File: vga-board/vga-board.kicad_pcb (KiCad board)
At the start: 2 copper layers, 141 x 95.2 mm, 44 parts, among them J1 Conn_02x20_Odd_Even, J2 Conn_02x20_Odd_Even, J3 DB15_Female_HighDensity, U1 74HC244, U10 74HC163, U11 74LS158, U12 74LS251, U13 74HC244, U14 74HC244, U15 74HC244, U16 GAL22V10, U17 GAL22V10, U18 GAL22V10, U19 74HC163, U2 74HC373, U20 74HC163, U21 74HC163, U22 74HC163, U23 74HC163, U3 74HC244, U4 74HC373, U5 74HC373, U6 74HC373, U7 74HC373, U8 71256SA12TPG, U9 74HC244, X1 40MHz

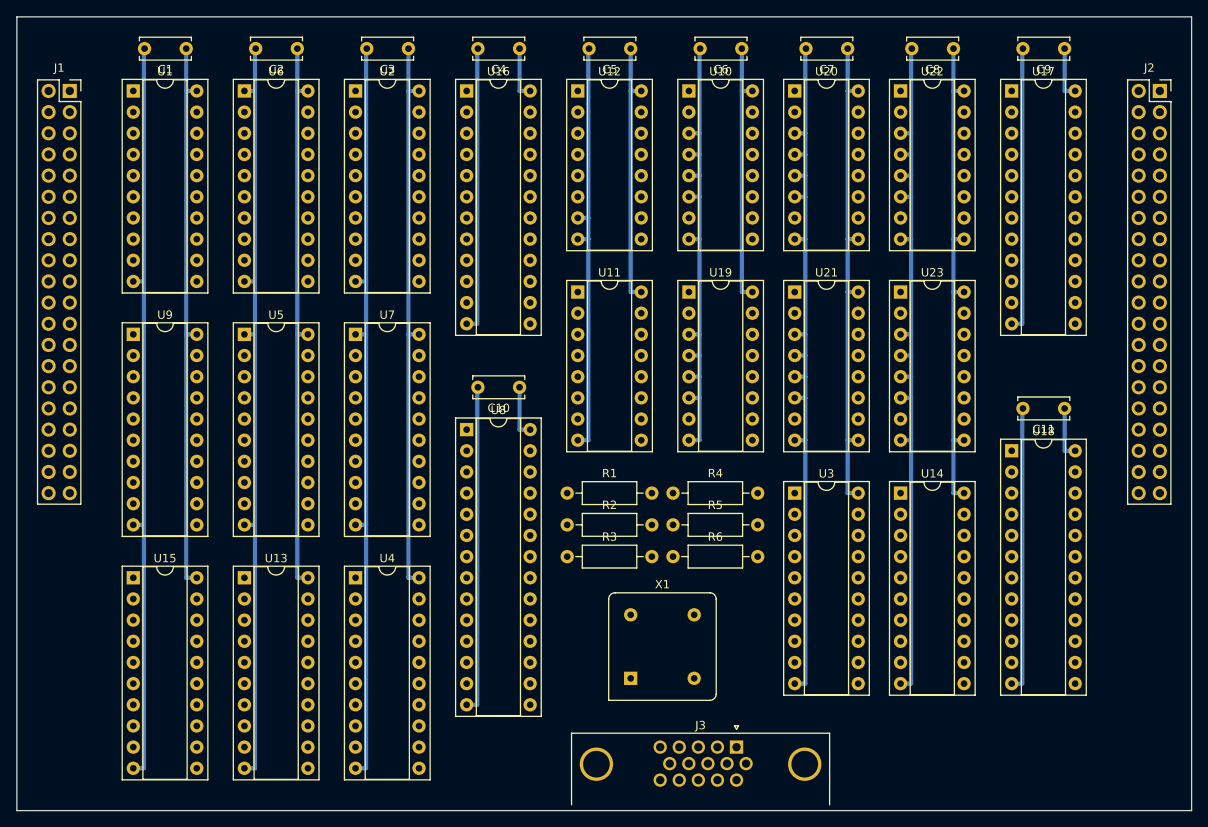
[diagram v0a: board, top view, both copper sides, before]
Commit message: Revert "More on layouts"
This reverts commit 3fc7c4d1a32f245eaa0a26aebed00be081417dbd.
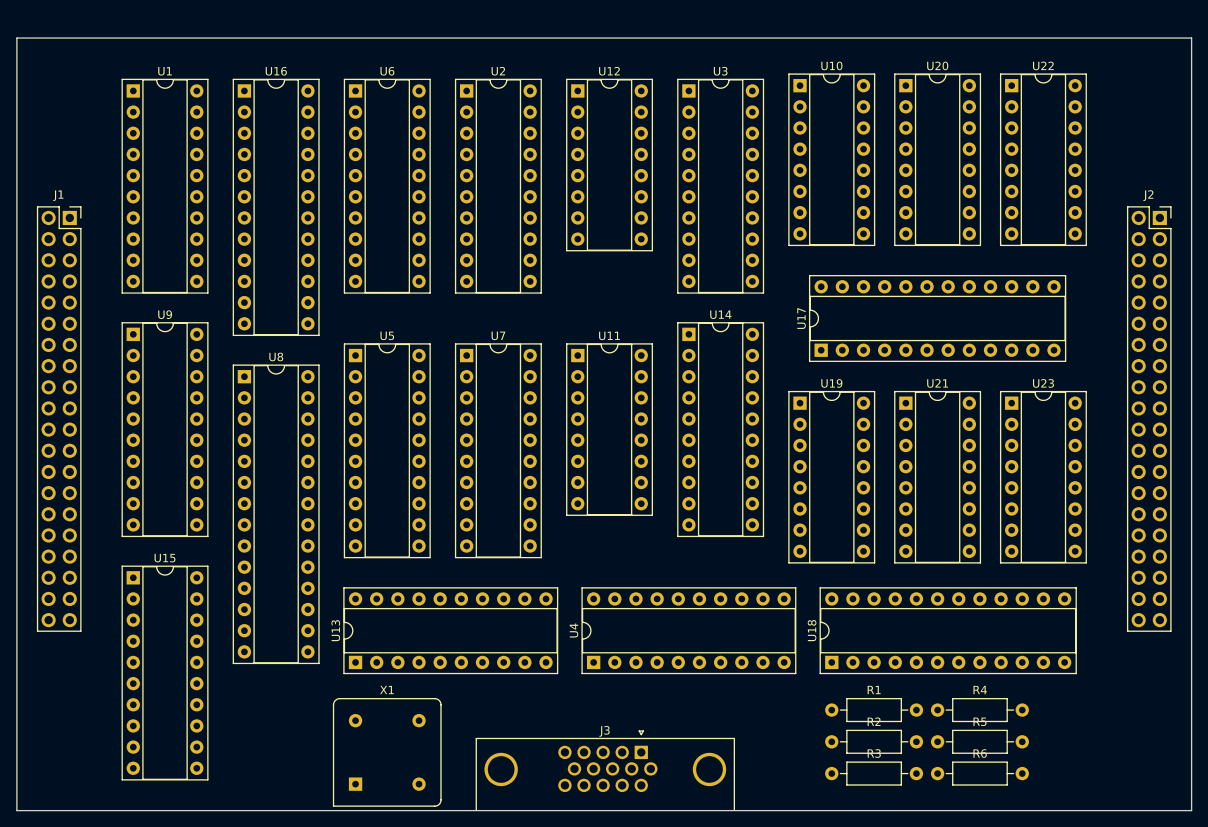
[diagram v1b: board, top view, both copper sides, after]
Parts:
- removed C1, C10, C11, C2, C3, C4, C5, C6, C7, C8, C9: 0.1uF, Capacitor_THT:C_Disc_D6.0mm_W2.5mm_P5.00mm
- moved U3 49.9 mm to (161.3, 48.3)
- moved R1 41.1 mm to (178.4, 122.6)
- moved R3 41.1 mm to (178.4, 130.2)
- moved R4 41.1 mm to (191.1, 122.6)
- moved R6 41.1 mm to (191.1, 130.2)
- moved R2 41.1 mm to (178.4, 126.4)
- moved R5 41.1 mm to (191.1, 126.4)
- moved U17 38.6 mm to (177.2, 79.4), turned to 90 degrees
- moved X1 35.4 mm to (121.3, 131.4)
- moved U18 33.3 mm to (178.4, 116.8), turned to 90 degrees
- moved U14 31.8 mm to (161.3, 77.5)
- moved U4 30.3 mm to (149.9, 116.8), turned to 90 degrees
- moved U8 27.4 mm to (108.0, 82.5)
- moved U16 26.7 mm to (108.0, 48.3)
- moved U19 18.9 mm to (174.6, 85.7)
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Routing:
- net GND: track 707.8 -> 0.00 mm
- net +5V: track 410.2 -> 0.00 mm
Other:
- board size 141 x 95.2 mm -> 141 x 92.7 mm

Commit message: More on layouts
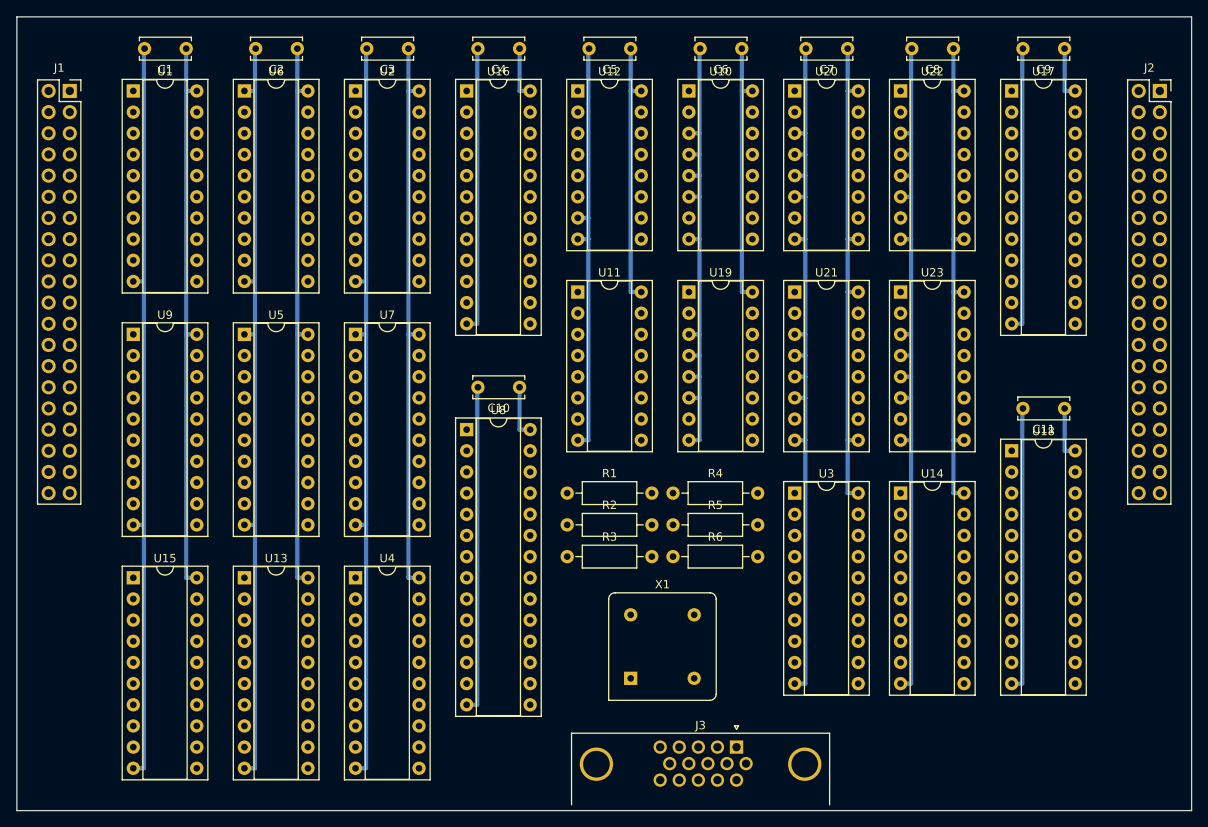
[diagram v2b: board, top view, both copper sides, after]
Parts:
- added C1: 0.1uF, Capacitor_THT:C_Disc_D6.0mm_W2.5mm_P5.00mm, F.Cu at (101.0, 43.2)
- added C10: 0.1uF, Capacitor_THT:C_Disc_D6.0mm_W2.5mm_P5.00mm, F.Cu at (141.0, 83.8)
- added C11: 0.1uF, Capacitor_THT:C_Disc_D6.0mm_W2.5mm_P5.00mm, F.Cu at (206.4, 86.4)
- added C2: 0.1uF, Capacitor_THT:C_Disc_D6.0mm_W2.5mm_P5.00mm, F.Cu at (114.3, 43.2)
- added C3: 0.1uF, Capacitor_THT:C_Disc_D6.0mm_W2.5mm_P5.00mm, F.Cu at (127.6, 43.2)
- added C4: 0.1uF, Capacitor_THT:C_Disc_D6.0mm_W2.5mm_P5.00mm, F.Cu at (141.0, 43.2)
- added C5: 0.1uF, Capacitor_THT:C_Disc_D6.0mm_W2.5mm_P5.00mm, F.Cu at (154.3, 43.2)
- added C6: 0.1uF, Capacitor_THT:C_Disc_D6.0mm_W2.5mm_P5.00mm, F.Cu at (167.6, 43.2)
- added C7: 0.1uF, Capacitor_THT:C_Disc_D6.0mm_W2.5mm_P5.00mm, F.Cu at (180.3, 43.2)
- added C8: 0.1uF, Capacitor_THT:C_Disc_D6.0mm_W2.5mm_P5.00mm, F.Cu at (193.0, 43.2)
- added C9: 0.1uF, Capacitor_THT:C_Disc_D6.0mm_W2.5mm_P5.00mm, F.Cu at (206.4, 43.2)
- moved U3 49.9 mm to (174.0, 96.5)
- moved R1 41.1 mm to (146.7, 96.5)
- moved R3 41.1 mm to (146.7, 104.1)
- moved R4 41.1 mm to (159.4, 96.5)
- moved R6 41.1 mm to (159.4, 104.1)
- moved R2 41.1 mm to (146.7, 100.3)
- moved R5 41.1 mm to (159.4, 100.3)
- moved U17 38.6 mm to (200.0, 48.3), turned to 0 degrees
- moved X1 35.4 mm to (154.3, 118.7)
- moved U18 33.3 mm to (200.0, 91.4), turned to 0 degrees
- moved U14 31.8 mm to (186.7, 96.5)
- moved U4 30.3 mm to (121.3, 106.7), turned to 0 degrees
- moved U8 27.4 mm to (134.6, 88.9)
- moved U16 26.7 mm to (134.6, 48.3)
- moved U19 18.9 mm to (161.3, 72.4)
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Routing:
- net GND: track 0.00 -> 707.8 mm
- net +5V: track 0.00 -> 410.2 mm
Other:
- board size 141 x 92.7 mm -> 141 x 95.2 mm
